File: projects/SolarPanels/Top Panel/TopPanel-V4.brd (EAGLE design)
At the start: 31 parts

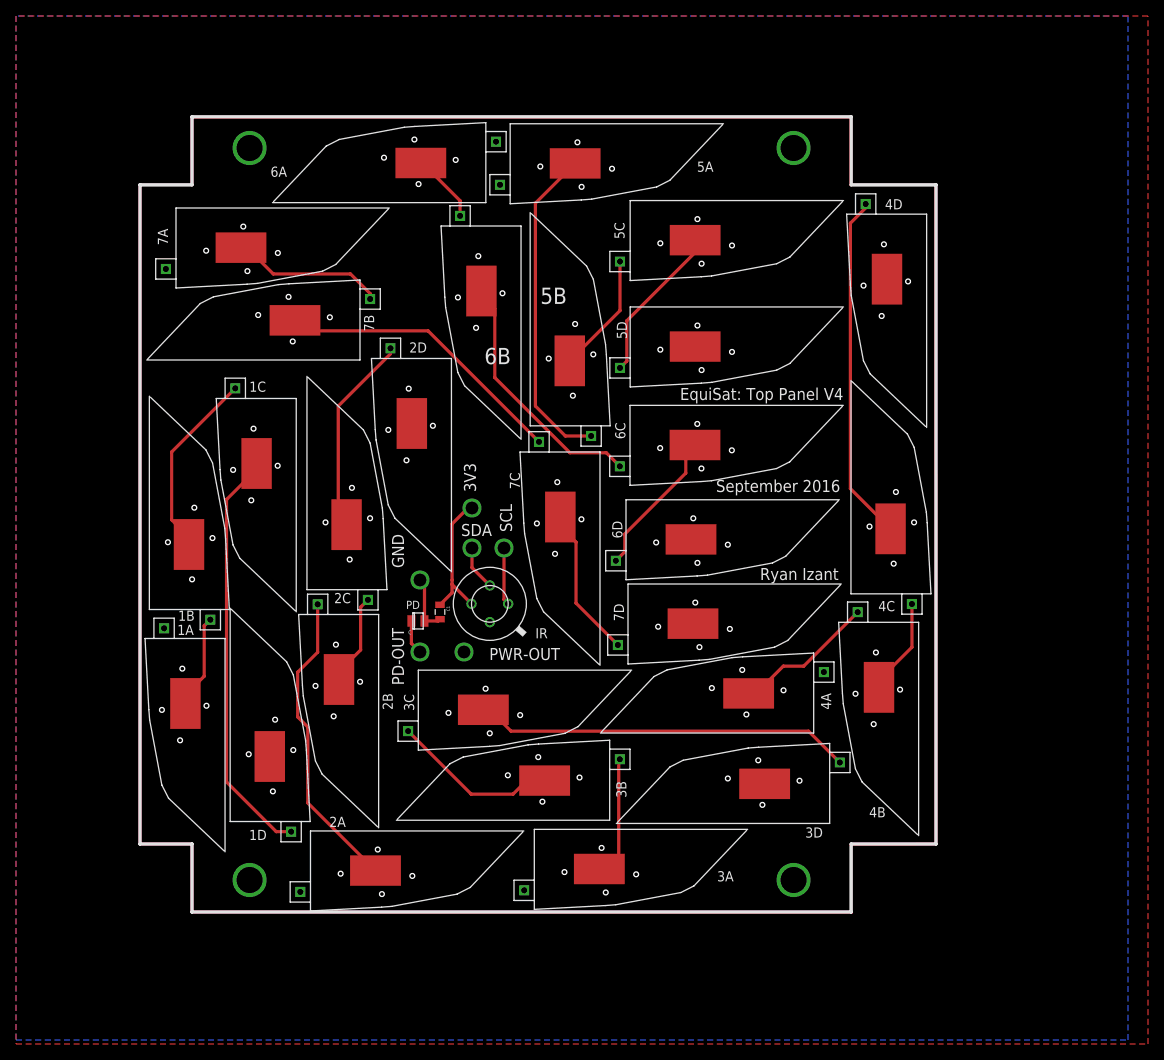
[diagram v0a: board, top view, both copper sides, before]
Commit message: Updated with processor test board V2
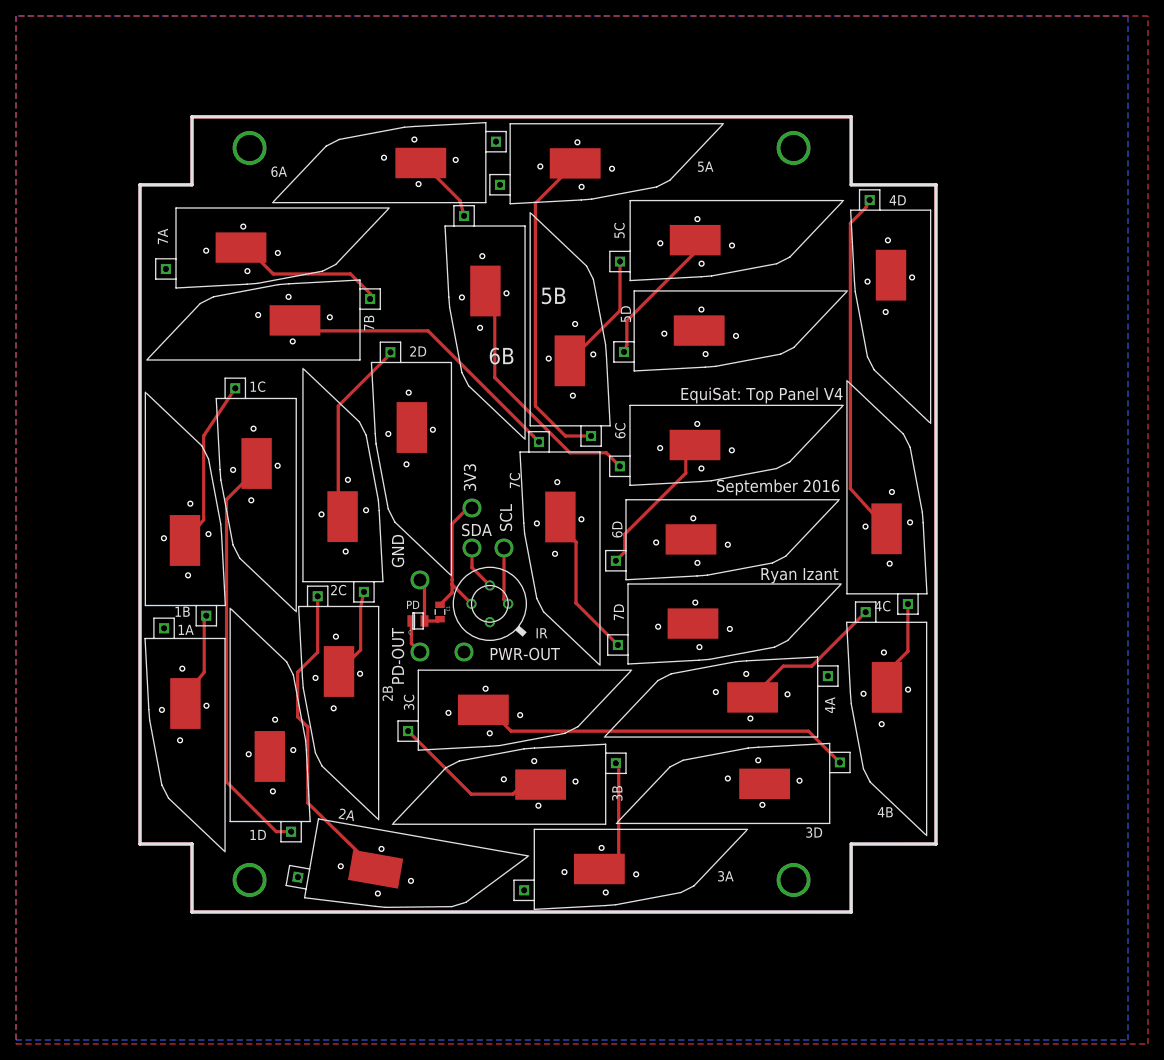
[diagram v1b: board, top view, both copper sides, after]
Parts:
- moved 5D 2.06 mm to (55.3, 77.6)
- moved 2A 1.80 mm to (15.8, 11.6), turned to 260 degrees
- moved 2C 1.12 mm to (13.9, 41.3)
- moved 2B 1.00 mm to (23.3, 38.2)
- moved 4B 1.00 mm to (91.8, 36.2)
- moved 1B 0.71 mm to (-5.83, 38.3)
- moved 3B 0.71 mm to (51.7, 11.0)
- moved 4A 0.71 mm to (78.2, 21.9)
- moved 4D 0.71 mm to (92.3, 87.7)
- moved 2D 0.50 mm to (32.4, 68.7)
- moved 4C 0.50 mm to (81.9, 39.8)
- moved 6B 0.50 mm to (41.6, 85.8)
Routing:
- net N$2: track 23.7 -> 21.1 mm
- net N$23: track 19.9 -> 17.6 mm
- net N$6: track 38.3 -> 39.2 mm
- net N$16: track 17.8 -> 18.6 mm
